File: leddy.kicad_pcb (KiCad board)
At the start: 4 copper layers, 86.8 x 60.8 mm, 82 parts, among them J1 hole 1, J2 hole 1, J3 hole 1, J4 hole 1, J5 umbrella support, J6 BARREL_JACK, J7 OPEN HARDWARE, J8 label_power-in, Q1 ZXMP6A13GTA, SW1 SW_DPST, U1 LT3518EFE#PBF, U2 74HC4017PW

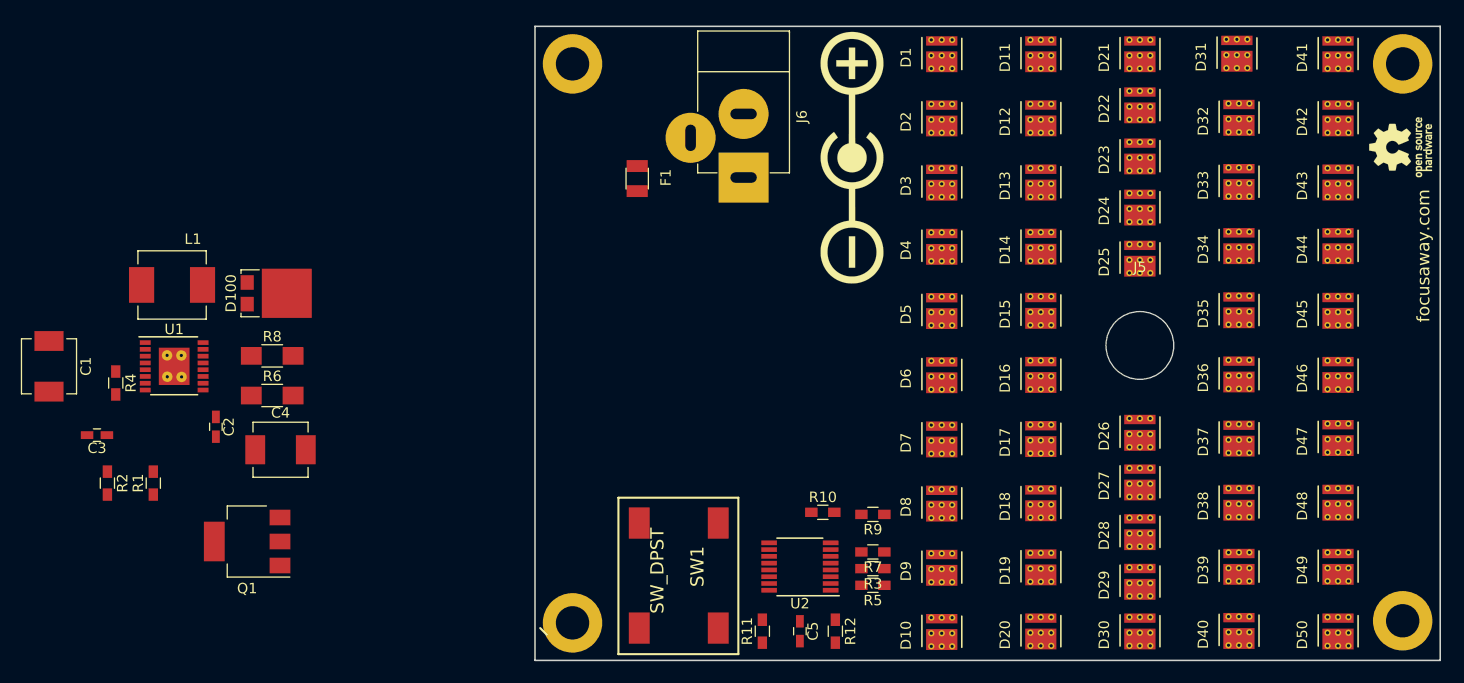
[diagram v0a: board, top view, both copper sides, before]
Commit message: started PCB layouting
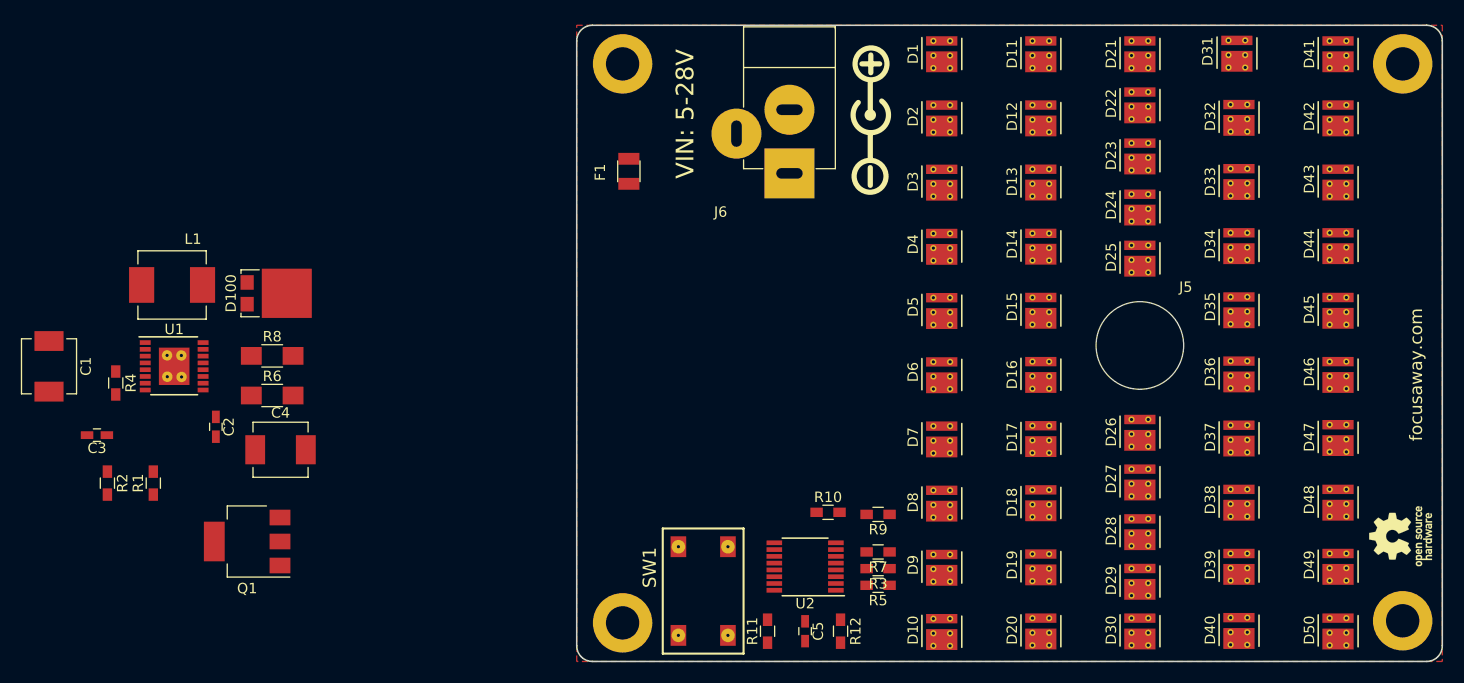
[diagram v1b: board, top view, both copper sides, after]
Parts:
- J5: footprint Mounting_Holes:MountingHole_6.5mm -> Mounting_Holes:MountingHole_8.4mm_M8
- J8: footprint Symbols:Polarity_Center_Positive_6mm_SilkScreen -> lib:Polarity_Center_Positive_3mm_SilkScreen
- SW1: value SW_DPST -> PTS645SM70SMTR92
- moved J7 37.3 mm to (207.0, 96.5)
- moved J1 4.80 mm to (132.4, 51.2)
- moved J2 4.80 mm to (132.4, 104.8)
- moved J8 4.49 mm to (156.0, 56.0)
- moved J6 4.42 mm to (148.4, 61.7)
- moved SW1 1.22 mm to (138.0, 100.5)
- moved F1 1.06 mm to (133.0, 61.5), turned to 90 degrees
- moved C5 0.50 mm to (149.9, 105.6)
- moved R10 0.50 mm to (152.1, 94.2)
- moved R11 0.50 mm to (146.3, 105.6)
- moved R12 0.50 mm to (153.3, 105.6)
- moved R3 0.50 mm to (156.9, 99.6)
- moved R5 0.50 mm to (156.9, 101.2)
- moved R7 0.50 mm to (156.9, 98.0)
- moved R9 0.50 mm to (156.9, 94.4)
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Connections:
- SW1 pad 1: Net-(SW1-Pad1) -> Net-(C5-Pad1)
- SW1 pad 3: Net-(C5-Pad1) -> Net-(SW1-Pad3)
- SW1 pad 4: Net-(SW1-Pad4) -> Net-(R12-Pad2)
- U2 pad 14: Net-(C5-Pad1) -> Net-(U2-Pad14)
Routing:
- added copper zone on F.Cu, net GND
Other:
- board size 86.8 x 60.8 mm -> 83 x 61 mm
- board text added: "VIN: 5-28V"
